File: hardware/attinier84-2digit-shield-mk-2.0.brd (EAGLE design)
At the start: 31 x 29 mm, 5 parts, among them IC1 TMP36, U1 ATTINIER84_SHIELD1551G

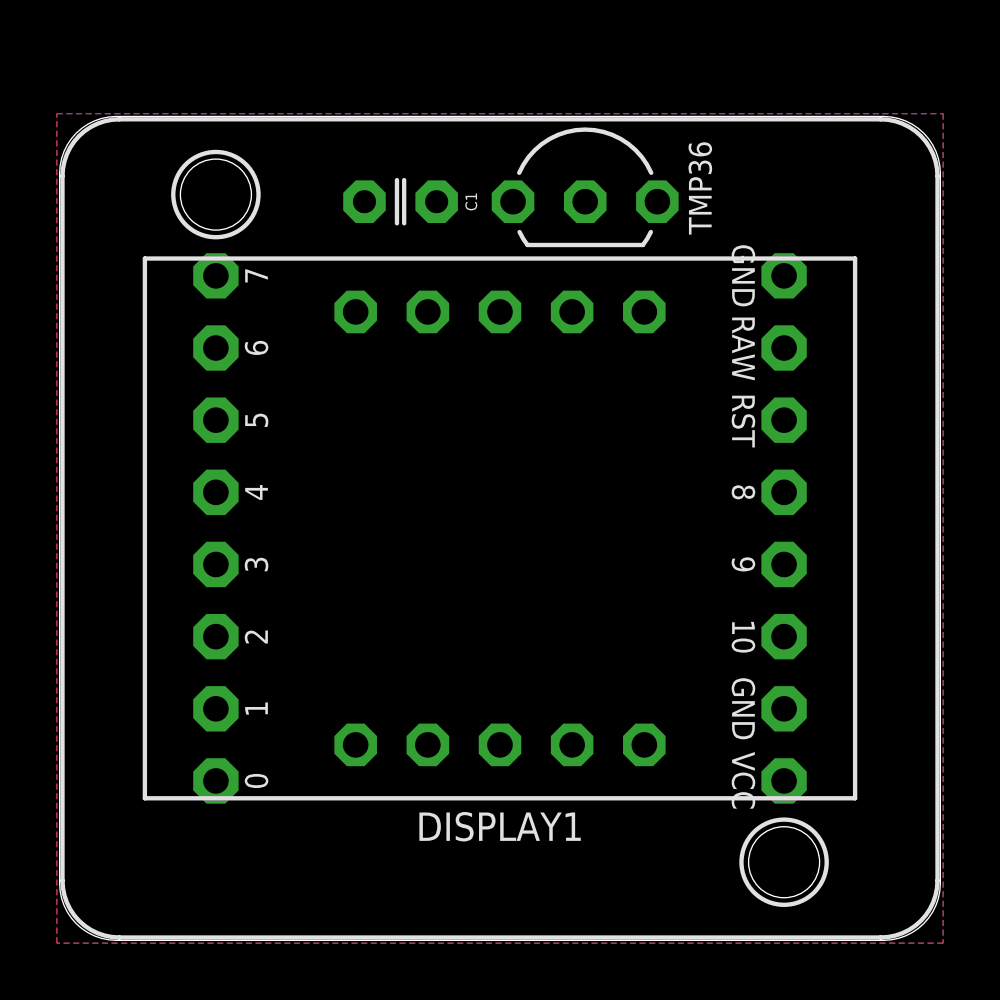
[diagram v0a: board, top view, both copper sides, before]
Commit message: temp shield with display done
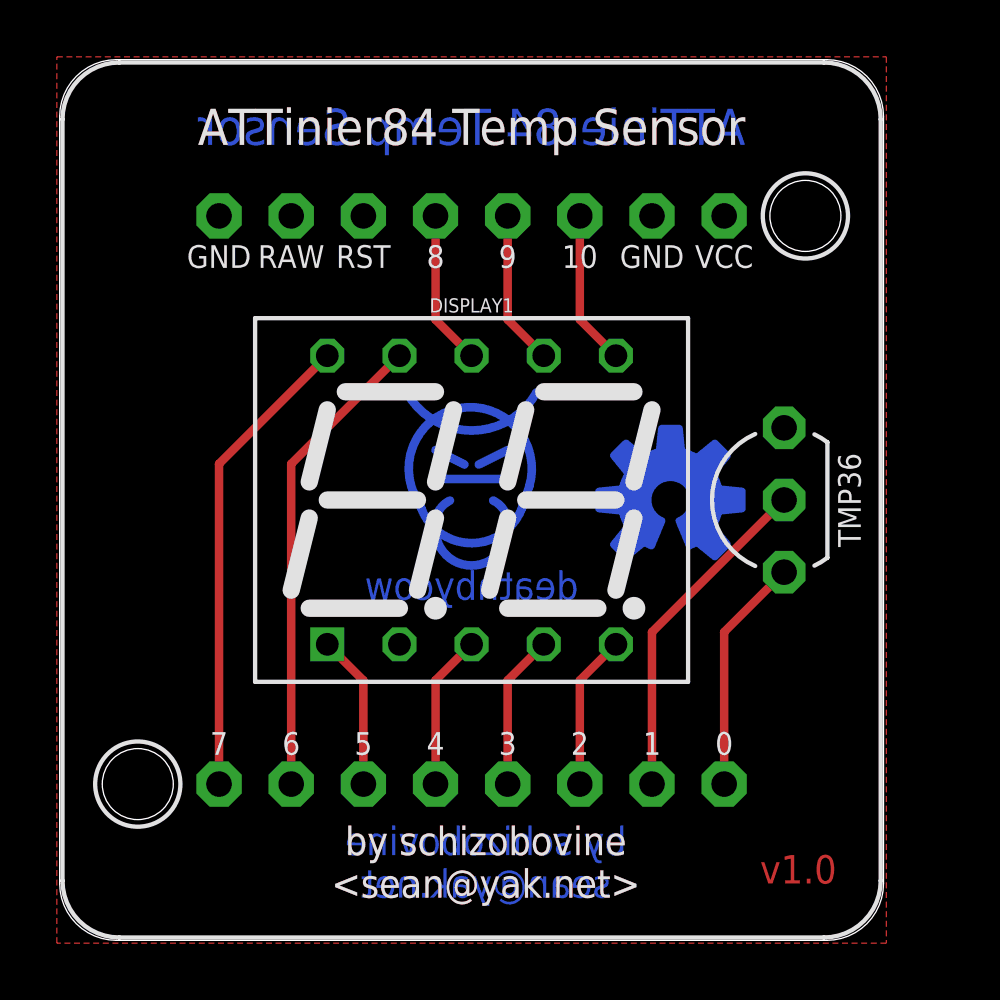
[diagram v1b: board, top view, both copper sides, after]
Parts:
- removed C1: 0.1uF, A_butts:C025-024X044
- added U$1: (no value), A_butts:CC-BY-SA-4.0-NO-URL
- added U$2: (no value), A_butts:COW_SMALL_METAL
- added U$3: (no value), A_butts:OSHWLOGO_BOT_0.2_A
- DISPLAY1: value 7SEG_2DIG19MM -> 7SEG_2DIG14MM; device A_butts:7SEG_2DIG_19MM -> A_butts:7SEG_2DIG_14MM
- moved FRAME1 29.0 mm to (29.0, 0.00), turned to 90 degrees
- moved IC1 12.6 mm to (25.5, 15.5), turned to 90 degrees
- moved DISPLAY1 1.41 mm to (14.5, 15.5)
- moved U1 1.41 mm to (14.5, 15.5), turned to 90 degrees
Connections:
- net GND: no longer C1.2
- net PA0: now also IC1.1; no longer DISPLAY1.1
- net PA1: now also IC1.2; no longer DISPLAY1.2
- net PA2: now also DISPLAY1.5; no longer DISPLAY1.3
- net PA4: now also DISPLAY1.3; no longer DISPLAY1.8
- net PA5: now also DISPLAY1.1; no longer DISPLAY1.9
- net PA6: now also DISPLAY1.9; no longer DISPLAY1.10
- net PA7: now also DISPLAY1.10; no longer IC1.2
- net PB0: now also DISPLAY1.6; no longer DISPLAY1.5
- net PB2: now also DISPLAY1.8; no longer DISPLAY1.6
- net VCC: no longer C1.1, IC1.1
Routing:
- net PA7: track 0.00 -> 16.7 mm
- net PA6: track 0.00 -> 16.7 mm
- net PA1: track 0.00 -> 11.9 mm
- net PA0: track 0.00 -> 8.33 mm
- net PB2: track 0.00 -> 5.45 mm
- net PB1: track 0.00 -> 5.45 mm
- net PB0: track 0.00 -> 5.45 mm
- net PA5: track 0.00 -> 5.45 mm
- net PA4: track 0.00 -> 5.45 mm
- net PA3: track 0.00 -> 5.45 mm
- net PA2: track 0.00 -> 5.45 mm
- removed copper zone on layer 16, net GND
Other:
- board size 31 x 29 mm -> 29 x 31 mm
- board text added: ">REVISION"
- board text added: "ATTinier84 Temp Sensor"
- board text added: "by schizobovine <sean@yak.net>"
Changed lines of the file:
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@@
 <setting verticaltext="up"/>
 </settings>
-<grid distance="0.5" unitdist="mm" unit="mm" style="lines" multiple="2" display="yes" altdistance="1" altunitdist="mil" altunit="mil"/>
+<grid distance="0.25" unitdist="mm" unit="mm" style="lines" multiple="2" display="yes" altdistance="1" altunitdist="mil" altunit="mil"/>
 <layers>
 <layer number="1" name="Top" color="4" fill="1" visible="yes" active="yes"/>
@@
 <board>
 <plain>
+<text x="14.5" y="28" size="1.27" layer="1" font="vector" ratio="15" align="bottom-center">ATTinier84 Temp Sensor</text>
+<text x="14.5" y="28" size="1.27" layer="21" font="vector" ratio="15" align="bottom-center">ATTinier84 Temp Sensor</text>
+<text x="26" y="2" size="1" layer="1" font="vector" ratio="16" align="bottom-center">&gt;REVISION</text>
+<text x="26" y="2" size="1" layer="21" font="vector" ratio="16" align="bottom-center">&gt;REVISION</text>
+<text x="26" y="2" size="1" layer="16" font="vector" ratio="16" rot="MR0" align="bottom-center">&gt;REVISION</text>
+<text x="26" y="2" size="1" layer="22" font="vector" ratio="16" rot="MR0" align="bottom-center">&gt;REVISION</text>
+<text x="14.5" y="28" size="1.27" layer="16" font="vector" ratio="15" rot="MR0" align="bottom-center">ATTinier84 Temp Sensor</text>
+<text x="14.5" y="28" size="1.27" layer="22" font="vector" ratio="15" rot="MR0" align="bottom-center">ATTinier84 Temp Sensor</text>
+<text x="15" y="1.5" size="1" layer="21" font="vector" ratio="16" align="bottom-center">by schizobovine
+&lt;sean@yak.net&gt;</text>
+<text x="15" y="1.5" size="1" layer="1" font="vector" ratio="16" align="bottom-center">by schizobovine
+&lt;sean@yak.net&gt;</text>
+<text x="15" y="1.5" size="1" layer="22" font="vector" ratio="16" rot="MR0" align="bottom-center">by schizobovine
+&lt;sean@yak.net&gt;</text>
+<text x="15" y="1.5" size="1" layer="16" font="vector" ratio="16" rot="MR0" align="bottom-center">by schizobovine
+&lt;sean@yak.net&gt;</text>
 </plain>
 <attributes>
+<attribute name="REVISION" value="v1.0"/>
 </attributes>
 <variantdefs>
@@
 </autorouter>
 <elements>
-<element name="FRAME1" library="A_butts" package="DUMMY" value="" x="0" y="0">
-<attribute name="VERSION" value="v01" x="13.97" y="-30.48" size="1.778" layer="27" display="off"/>
-<attribute name="DESIGNER" value="Nobody" x="13.97" y="-30.48" size="1.778" layer="27" display="off"/>
+<element name="FRAME1" library="A_butts" package="DUMMY" value="" x="29" y="0" rot="R90">
+<attribute name="VERSION" value="v01" x="59.48" y="13.97" size="1.778" layer="27" rot="R90" display="off"/>
+<attribute name="DESIGNER" value="Nobody" x="59.48" y="13.97" size="1.778" layer="27" rot="R90" display="off"/>
 </element>
-<element name="U1" library="A_butts" package="ATTINIER84_SHIELD2" value="ATTINIER84_SHIELD1551G" x="15.5" y="14.5"/>
-<element name="DISPLAY1" library="A_butts" package="7SEG_2DIG_19MM" value="7SEG_2DIG19MM" x="15.5" y="14.5"/>
-<element name="IC1" library="A_butts" package="TO-92-AMMO" value="TMP36" x="18.5" y="26" smashed="yes">
-<attribute name="VALUE" x="22.151" y="26.5" size="0.8" layer="21" font="vector" ratio="12" rot="R90" align="top-center"/>
+<element name="U1" library="A_butts" package="ATTINIER84_SHIELD2" value="ATTINIER84_SHIELD1551G" x="14.5" y="15.5" rot="R90"/>
+<element name="DISPLAY1" library="A_butts" package="7SEG_2DIG_14MM" value="7SEG_2DIG14MM" x="14.5" y="15.5"/>
+<element name="IC1" library="A_butts" package="TO-92-AMMO" value="TMP36" x="25.5" y="15.5" smashed="yes" rot="R90">
+<attribute name="VALUE" x="27.401" y="15.5" size="0.8" layer="21" font="vector" ratio="12" rot="R90" align="top-center"/>
 </element>
-<element name="C1" library="A_butts" package="C025-024X044" value="0.1uF" x="12" y="26" rot="R180"/>
+<element name="U$1" library="A_butts" package="CC-BY-SA-4.0-NO-URL" value="" x="6" y="15.5" rot="MR0"/>
+<element name="U$2" library="A_butts" package="COW_SMALL_METAL" value="" x="14.5" y="16.75" rot="MR0"/>
+<element name="U$3" library="A_butts" package="OSHWLOGO_BOT_0.2_A" value="" x="21.5" y="15.5"/>
 </elements>
 <signals>
@@
 <contactref element="U1" pad="GND@1"/>
 <polygon width="0.1524" layer="1">
+<vertex x="29.1" y="-0.1"/>
 <vertex x="-0.1" y="-0.1"/>
-<vertex x="-0.1" y="29.1"/>
-<vertex x="31.1" y="29.1"/>
-<vertex x="31.1" y="-0.1"/>
-</polygon>
-<polygon width="0.1524" layer="16">
-<vertex x="-0.1" y="-0.1"/>
-<vertex x="-0.1" y="29.1"/>
-<vertex x="31.1" y="29.1"/>
-<vertex x="31.1" y="-0.1"/>
+<vertex x="-0.1" y="31.1"/>
+<vertex x="29.1" y="31.1"/>
 </polygon>
 <contactref element="IC1" pad="3"/>
-<contactref element="C1" pad="2"/>
 </signal>
 <signal name="VCC">
 <contactref element="U1" pad="VCC"/>
-<contactref element="IC1" pad="1"/>
-<contactref element="C1" pad="1"/>
-<wire x1="13.27" y1="26" x2="15.96" y2="26" width="0" layer="19" extent="1-1"/>
-<wire x1="25.5" y1="5.61" x2="15.96" y2="26" width="0" layer="19" extent="1-1"/>
 </signal>
 <signal name="PA7">
 <contactref element="U1" pad="PA7"/>
-<contactref element="IC1" pad="2"/>
-<wire x1="5.5" y1="23.39" x2="18.5" y2="26" width="0" layer="19" extent="1-1"/>
+<contactref element="DISPLAY1" pad="10"/>
+<wire x1="5.61" y1="5.5" x2="5.61" y2="16.77" width="0.3" layer="1"/>
+<wire x1="5.61" y1="16.77" x2="9.42" y2="20.58" width="0.3" layer="1"/>
 </signal>
 <signal name="PA6">
 <contactref element="U1" pad="PA6"/>
-<contactref element="DISPLAY1" pad="10"/>
-<wire x1="5.5" y1="20.85" x2="10.42" y2="22.12" width="0" layer="19" extent="1-1"/>
+<contactref element="DISPLAY1" pad="9"/>
+<wire x1="8.15" y1="5.5" x2="8.15" y2="16.77" width="0.3" layer="1"/>
+<wire x1="8.15" y1="16.77" x2="11.96" y2="20.58" width="0.3" layer="1"/>
 </signal>
 <signal name="PA5">
 <contactref element="U1" pad="PA5"/>
-<contactref element="DISPLAY1" pad="9"/>
-<wire x1="5.5" y1="18.31" x2="12.96" y2="22.12" width="0" layer="19" extent="1-1"/>
+<contactref element="DISPLAY1" pad="1"/>
+<wire x1="10.69" y1="5.5" x2="10.69" y2="9.15" width="0.3" layer="1"/>
+<wire x1="10.69" y1="9.15" x2="9.42" y2="10.42" width="0.3" layer="1"/>
 </signal>
 <signal name="PA4">
 <contactref element="U1" pad="PA4"/>
-<contactref element="DISPLAY1" pad="8"/>
-<wire x1="5.5" y1="15.77" x2="15.5" y2="22.12" width="0" layer="19" extent="1-1"/>
+<contactref element="DISPLAY1" pad="3"/>
+<wire x1="13.23" y1="5.5" x2="13.23" y2="9.15" width="0.3" layer="1"/>
+<wire x1="13.23" y1="9.15" x2="14.5" y2="10.42" width="0.3" layer="1"/>
 </signal>
 <signal name="PA3">
 <contactref element="U1" pad="PA3"/>
 <contactref element="DISPLAY1" pad="4"/>
-<wire x1="5.5" y1="13.23" x2="18.04" y2="6.88" width="0" layer="19" extent="1-1"/>
+<wire x1="15.77" y1="5.5" x2="15.77" y2="9.15" width="0.3" layer="1"/>
+<wire x1="15.77" y1="9.15" x2="17.04" y2="10.42" width="0.3" layer="1"/>
 </signal>
 <signal name="PA2">
 <contactref element="U1" pad="PA2"/>
-<contactref element="DISPLAY1" pad="3"/>
-<wire x1="5.5" y1="10.69" x2="15.5" y2="6.88" width="0" layer="19" extent="1-1"/>
+<contactref element="DISPLAY1" pad="5"/>
+<wire x1="18.31" y1="5.5" x2="18.31" y2="9.15" width="0.3" layer="1"/>
+<wire x1="18.31" y1="9.15" x2="19.58" y2="10.42" width="0.3" layer="1"/>
 </signal>
 <signal name="PA1">
 <contactref element="U1" pad="PA1"/>
-<contactref element="DISPLAY1" pad="2"/>
-<wire x1="5.5" y1="8.15" x2="12.96" y2="6.88" width="0" layer="19" extent="1-1"/>
+<contactref element="IC1" pad="2"/>
+<wire x1="20.85" y1="5.5" x2="20.85" y2="10.85" width="0.3" layer="1"/>
+<wire x1="20.85" y1="10.85" x2="25.5" y2="15.5" width="0.3" layer="1"/>
 </signal>
 <signal name="PA0">
 <contactref element="U1" pad="PA0"/>
-<contactref element="DISPLAY1" pad="1"/>
-<wire x1="5.5" y1="5.61" x2="10.42" y2="6.88" width="0" layer="19" extent="1-1"/>
+<contactref element="IC1" pad="1"/>
+<wire x1="23.39" y1="5.5" x2="23.39" y2="10.85" width="0.3" layer="1"/>
+<wire x1="23.39" y1="10.85" x2="25.5" y2="12.96" width="0.3" layer="1"/>
 </signal>
 <signal name="PB0">
 <contactref element="U1" pad="PB0"/>
-<contactref element="DISPLAY1" pad="5"/>
-<wire x1="20.58" y1="6.88" x2="25.5" y2="10.69" width="0" layer="19" extent="1-1"/>
+<contactref element="DISPLAY1" pad="6"/>
+<wire x1="18.31" y1="25.5" x2="18.31" y2="21.85" width="0.3" layer="1"/>
+<wire x1="18.31" y1="21.85" x2="19.58" y2="20.58" width="0.3" layer="1"/>
 </signal>
 <signal name="PB1">
 <contactref element="U1" pad="PB1"/>
 <contactref element="DISPLAY1" pad="7"/>
-<wire x1="18.04" y1="22.12" x2="25.5" y2="13.23" width="0" layer="19" extent="1-1"/>
+<wire x1="15.77" y1="25.5" x2="15.77" y2="21.85" width="0.3" layer="1"/>
+<wire x1="15.77" y1="21.85" x2="17.04" y2="20.58" width="0.3" layer="1"/>
 </signal>
 <signal name="PB2">
 <contactref element="U1" pad="PB2"/>
-<contactref element="DISPLAY1" pad="6"/>
-<wire x1="20.58" y1="22.12" x2="25.5" y2="15.77" width="0" layer="19" extent="1-1"/>
+<contactref element="DISPLAY1" pad="8"/>
+<wire x1="13.23" y1="25.5" x2="13.23" y2="21.85" width="0.3" layer="1"/>
+<wire x1="13.23" y1="21.85" x2="14.5" y2="20.58" width="0.3" layer="1"/>
 </signal>
 </signals>
 </board>
 </drawing>
+<compatibility>
+<note version="6.3" minversion="6.2.2" severity="warning">
+Since Version 6.2.2 text objects can contain more than one line,
+which will not be processed correctly with this version.
+</note>
+</compatibility>
 </eagle>
